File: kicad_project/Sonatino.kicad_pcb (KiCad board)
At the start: 4 copper layers, 65 x 30 mm, 129 parts, among them J2 Conn_02x09_Odd_Even, J3 USB_C_Receptacle_USB2.0, J4 Conn_01x01, J5 AudioJack4, J6 Conn_01x02, J7 Conn_01x02, Q1 DMP2104LP, Q2 DMP2104LP, Q3 HSCC8233, Q4 TPM3134NX3, Q5 DMP2104LP, SW1 SW_Push, SW2 SW_Push, SW3 SW_DIP_x02, U1 MAX98357A, U10 FSA2269, U11 TC7WH08FK,LJ(CT, U13 WM8524, U14 MAX4467, U15 WM8782, U16 TPA6132A2RTE, U2 ESP32-S3-WROOM-1U, U3 SRV05-4, U4 TP4056, U5 DW01x, U6 NCP167BMX330TBG, U7 NCP167BMX330TBG, U8 SN74LVC1G14DCKR, U9 FSA2269

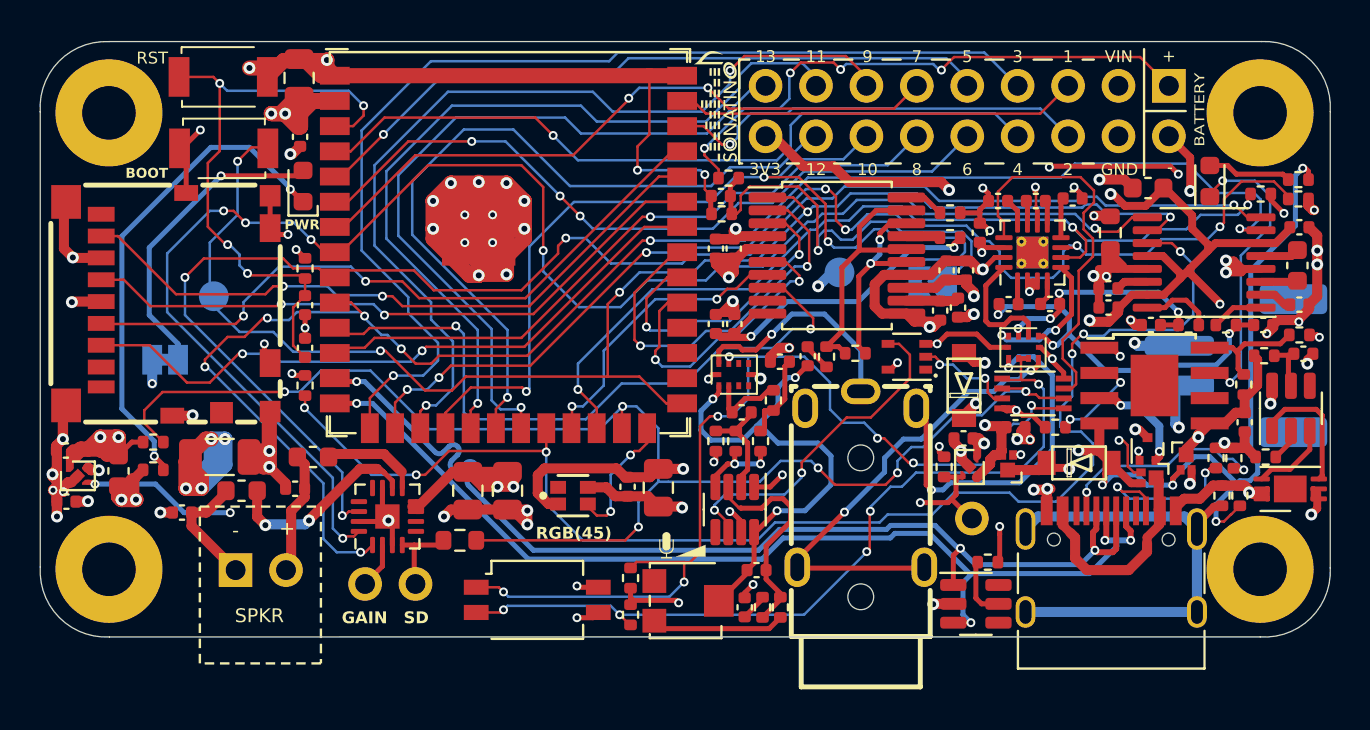
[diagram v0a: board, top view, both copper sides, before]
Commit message: Initial commit
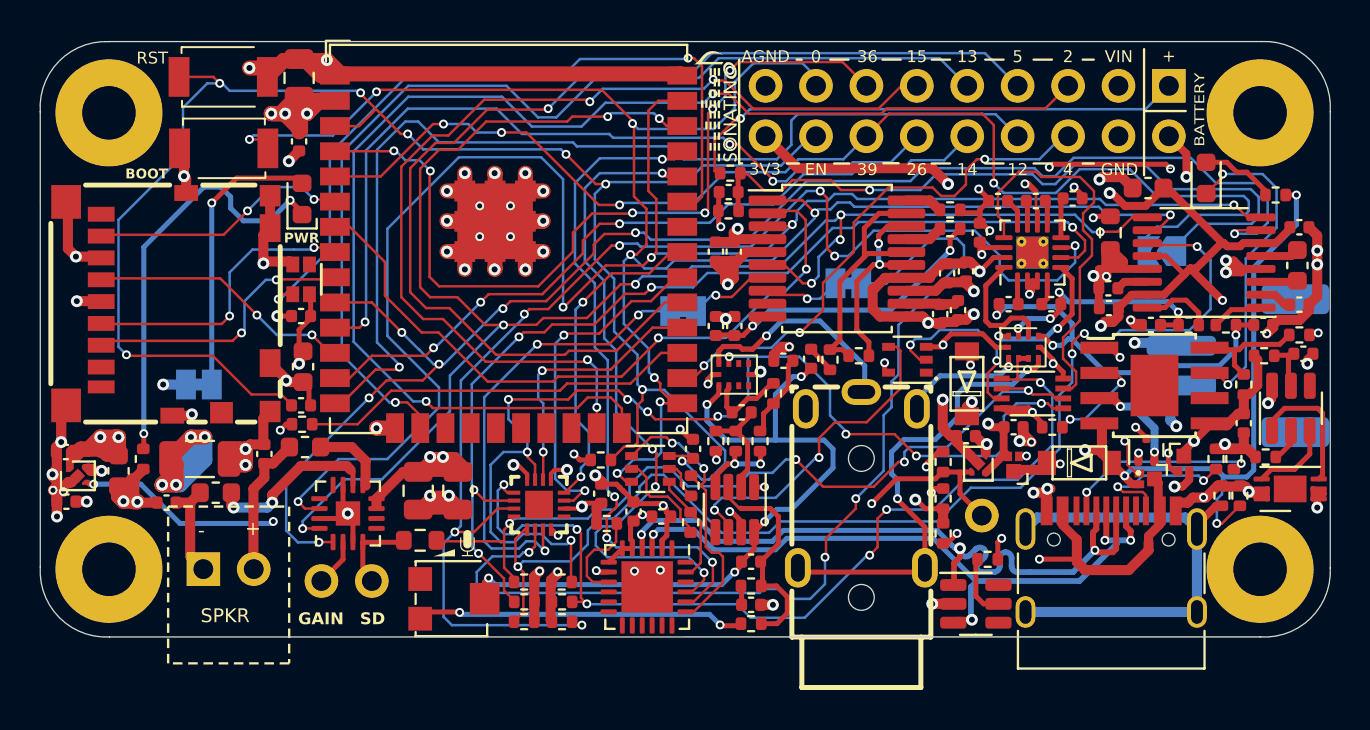
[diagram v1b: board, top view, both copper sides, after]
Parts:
- removed C47: 0.1uF, Capacitor_SMD:C_0402_1005Metric
- removed Card2: TF-008, Custom:TF-SMD_TF-008
- removed J4: Conn_01x01, Connector_PinHeader_2.54mm:PinHeader_1x01_P2.54mm_Vertical
- removed R19: 680K, Resistor_SMD:R_0603_1608Metric
- removed R4, R5, R8: 10K, Resistor_SMD:R_0402_1005Metric
- removed SW3: SW_DIP_x02, Button_Switch_SMD:SW_DIP_SPSTx02_Slide_Omron_A6H-2101_W6.15mm_P1.27mm
- removed TP1, TP2: TestPoint, TestPoint:TestPoint_Pad_D1.5mm
- added C17: 0.1uF, Capacitor_SMD:C_0402_1005Metric, F.Cu at (140.6, 46.6)
- added C48: 0.1uF, Capacitor_SMD:C_0402_1005Metric, F.Cu at (160.3, 53.3)
- added C49: 0.1uF, Capacitor_SMD:C_0402_1005Metric, F.Cu at (158.8, 56.7)
- added C50: 4.7uF, Capacitor_SMD:C_0402_1005Metric, F.Cu at (157.3, 56.5)
- added Card1: TF-008, Custom:TF-SMD_TF-008, F.Cu at (133.9, 46.0)
- added J8: Conn_01x01, Connector_PinHeader_2.54mm:PinHeader_1x01_P2.54mm_Vertical, F.Cu at (174.9, 56.7)
- added JP3: SolderJumper_2_Bridged, Jumper:SolderJumper-2_P1.3mm_Bridged_Pad1.0x1.5mm, B.Cu at (159.8, 46.4)
- added JP4: SolderJumper_2_Open, Jumper:SolderJumper-2_P1.3mm_Open_TrianglePad1.0x1.5mm, B.Cu at (184.0, 43.3)
- added Q6: MMDT3052DW 5G, Package_TO_SOT_SMD:SOT-363_SC-70-6, F.Cu at (158.2, 54.3)
- added R38: 22K, Resistor_SMD:R_0402_1005Metric, F.Cu at (172.9, 57.5)
- added R39: 47K, Resistor_SMD:R_0402_1005Metric, F.Cu at (172.9, 55.8)
- added R40: 150K, Resistor_SMD:R_0402_1005Metric, F.Cu at (162.1, 41.3)
- added R41: 470K, Resistor_SMD:R_0402_1005Metric, F.Cu at (162.2, 39.4)
- added R45: 10K, Resistor_SMD:R_0402_1005Metric, F.Cu at (151.8, 62.0)
- added R46: 10K, Resistor_SMD:R_0402_1005Metric, F.Cu at (151.8, 60.0)
- added R47: 10K, Resistor_SMD:R_0402_1005Metric, F.Cu at (153.8, 62.0)
- added R48: 10K, Resistor_SMD:R_0402_1005Metric, F.Cu at (151.8, 61.0)
- added R49: 10K, Resistor_SMD:R_0402_1005Metric, F.Cu at (153.8, 61.0)
- added R50: 10K, Resistor_SMD:R_0402_1005Metric, F.Cu at (153.7, 60.0)
- added U12: MAX98357A, Package_DFN_QFN:TQFN-16-1EP_3x3mm_P0.5mm_EP1.23x1.23mm, F.Cu at (143.0, 56.5)
- added U18: 74AHC595, Custom:X1-QFN-16-EP_L2.5-W2.5-P0.40-BL-EP1.4, F.Cu at (152.6, 56.1)
- C14: value 10uF -> 220pF; footprint Capacitor_SMD:C_0805_2012Metric -> Capacitor_SMD:C_0402_1005Metric
- C15: value 100nF -> 0.1uF; footprint Capacitor_SMD:C_0402_1005Metric -> Capacitor_SMD:C_0805_2012Metric
- C16: value 0.1uF -> 10uF
- C18: value 220pF -> 22uF; footprint Capacitor_SMD:C_0402_1005Metric -> Capacitor_SMD:C_0603_1608Metric
- C19: value 220pF -> 1uF
- C4: value 1uF -> 220pF
- C46: value 22uF -> 0.1uF; footprint Capacitor_SMD:C_0805_2012Metric -> Capacitor_SMD:C_0402_1005Metric
- JP2: value SolderJumper_2_Open -> SolderJumper_2_Bridged; footprint Jumper:SolderJumper-2_P1.3mm_Open_TrianglePad1.0x1.5mm -> Jumper:SolderJumper-2_P1.3mm_Bridged_Pad1.0x1.5mm
- Q1, Q2: footprint Custom:Diodes_DFN1411-3 -> CustomLibrary:Diodes_DFN1411-3
- Q4: value TPM3134NX3 -> DMP2104LP; footprint Package_TO_SOT_SMD:SOT-723 -> Custom:Diodes_DFN1411-3
- Q5: value DMP2104LP -> TPM3134NX3; footprint Custom:Diodes_DFN1411-3 -> Package_TO_SOT_SMD:SOT-723
- R3: value 10K -> 680K; footprint Resistor_SMD:R_0402_1005Metric -> Resistor_SMD:R_0603_1608Metric
- R34: value 150K -> 10K
- R35: value 470K -> 10K
- R37: value 100K -> 1K
- R6: value 10K -> 100K
- U1: value MAX98357A -> ESP32-WROOM-E; footprint Package_DFN_QFN:TQFN-16-1EP_3x3mm_P0.5mm_EP1.23x1.23mm -> Espressif:ESP32-WROOM-32UE
- U2: value ESP32-S3-WROOM-1U -> CP2102N-Axx-xQFN24; footprint Espressif:ESP32-S3-WROOM-1U -> Package_DFN_QFN:QFN-24-1EP_4x4mm_P0.5mm_EP2.6x2.6mm
- moved C19 31.9 mm to (162.1, 40.4)
- moved C15 21.3 mm to (146.5, 55.4), turned to -90 degrees
- moved R36 20.2 mm to (155.7, 53.9)
- moved U2 18.8 mm to (158.0, 60.2), turned to -90 degrees
- moved R7 18.2 mm to (175.2, 58.9), turned to 180 degrees
- moved D1 17.5 mm to (140.6, 44.8), turned to -90 degrees
- moved R34 17.5 mm to (160.2, 57.0), turned to 90 degrees
- moved R37 17.2 mm to (156.0, 57.0), turned to 180 degrees
- moved C14 17.2 mm to (133.8, 56.0), turned to 0 degrees
- moved R6 16.8 mm to (172.9, 54.0), turned to -90 degrees
- moved U1 15.1 mm to (151.1, 42.9), turned to 0 degrees
- moved R3 14.3 mm to (146.6, 57.9)
- moved R35 13.8 mm to (160.2, 55.1), turned to 90 degrees
- moved R28 11.8 mm to (148.2, 60.9)
- moved J7 8.18 mm to (135.7, 59.4)
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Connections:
- C14 pad 2: +5V -> Net-(J7-Pin_1)
- C15 pad 1: GND -> +5V
- C15 pad 2: Net-(JP2-A) -> GND
- C16 pad 1: +5V -> GND
- C16 pad 2: GND -> +5V
- C18 pad 1: Net-(J6-Pin_2) -> +3.3V
- C19 pad 2: Net-(J6-Pin_1) -> Net-(JP4-A)
- C4 pad 1: GND -> Net-(J7-Pin_2)
- C4 pad 2: /EN -> GND
- C46 pad 1: +3.3V -> GND
- C46 pad 2: GND -> +3.3V
- D2 pad 1: /USB & Power/VCC -> Net-(D2-K)
- D2 pad 2: Net-(D2-A) -> /VIN
- D3 pad 1: Net-(D2-A) -> /USB & Power/VCC
- D3 pad 2: /VIN -> Net-(D2-K)
- FB1 pad 1: Net-(U1-OUT-) -> Net-(U12-OUT-)
- FB1 pad 2: Net-(J6-Pin_1) -> Net-(J7-Pin_1)
- FB2 pad 1: Net-(J6-Pin_2) -> Net-(J7-Pin_2)
- FB2 pad 2: Net-(U1-OUT+) -> Net-(U12-OUT+)
- J2 pad 10: /GPIO6 -> /GPIO14
- J2 pad 11: /GPIO7 -> /GPIO15
- J2 pad 12: /GPIO8 -> /GPIO26
- J2 pad 13: /GPIO9 -> /GPIO36
- J2 pad 14: /GPIO10 -> /GPIO39
- J2 pad 15: /GPIO11 -> /BOOT/MCLK
- J2 pad 16: /GPIO12 -> /EN
- J2 pad 17: /GPIO13 -> GNDA
- J2 pad 5: /GPIO1 -> /GPIO2
- J2 pad 6: /GPIO2 -> /GPIO4
- J2 pad 7: /GPIO3 -> /GPIO5
- J2 pad 8: /GPIO4 -> /GPIO12
- J2 pad 9: /GPIO5 -> /GPIO13
- J3 pad A4: Net-(Q5-D) -> /USB & Power/VBUS
- J3 pad A6: /D+ -> /USB & Power/D+
- J3 pad A7: /D- -> /USB & Power/D-
- J3 pad A9: Net-(Q5-D) -> /USB & Power/VBUS
- J3 pad B4: Net-(Q5-D) -> /USB & Power/VBUS
- J3 pad B6: /D+ -> /USB & Power/D+
- J3 pad B7: /D- -> /USB & Power/D-
- J3 pad B9: Net-(Q5-D) -> /USB & Power/VBUS
- JP2 pad 2: /GPIO10 -> /ADC_RATE
- Q1 pad 1: Net-(D2-A) -> Net-(D2-K)
- Q4 pad 1: /USB & Power/VCC -> /VIN
- Q4 pad 2: Net-(Q4-S) -> Net-(D2-K)
- Q4 pad 3: GND -> /USB & Power/VBUS
- Q5 pad 1: /VIN -> /USB & Power/VCC
- Q5 pad 2: Net-(D2-A) -> Net-(Q5-S)
- Q5 pad 3: Net-(Q5-D) -> GND
- R12 pad 2: Net-(D2-A) -> Net-(D2-K)
- R13 pad 1: Net-(D2-A) -> Net-(D2-K)
- R2 pad 1: /~{MUTE} -> Net-(U1-GPIO16)
- R3 pad 1: +3.3V -> Net-(J6-Pin_2)
- R34 pad 1: /BAT+ -> Net-(Q6-B1)
- R34 pad 2: Net-(JP2-A) -> /USB & Power/DTR
- R35 pad 1: Net-(JP2-A) -> Net-(Q6-B2)
- R35 pad 2: GND -> /USB & Power/RTS
- R36 pad 1: Net-(D2-A) -> /EN
- R36 pad 2: Net-(U3-VP) -> +3.3V
- R37 pad 1: +5V -> Net-(U2-~{RST})
- R37 pad 2: /USB & Power/EN_REG -> +3.3V
- R6 pad 1: GND -> +5V
- R6 pad 2: /MIC_LINE_SELECT -> /USB & Power/EN_REG
- R7 pad 1: /HP_LINE_SELECT -> Net-(D2-K)
- R7 pad 2: GND -> Net-(U3-VP)
- SW2 pad 2: /MCLK -> /BOOT/MCLK
- U1 pad 1: /DAT_DAC -> GND
- U1 pad 10: Net-(U1-OUT-) -> /DAT_DAC
- U1 pad 11: GND -> /GPIO26
- U1 pad 12: (no net) -> /CLK
- U1 pad 13: (no net) -> /GPIO14
- U1 pad 14: /LRCLK_DAC -> /GPIO12
- U1 pad 16: /BCLK_DAC -> /GPIO13
- U1 pad 17: GND -> unconnected-(U1-NC-Pad17)
- U1 pad 2: Net-(J7-Pin_1) -> +3.3V
- U1 pad 3: GND -> /EN
- U1 pad 4: Net-(J7-Pin_2) -> /GPIO36
- U1 pad 5: (no net) -> /GPIO39
- U1 pad 6: (no net) -> /D0
- U1 pad 7: +5V -> /DAT_ADC
- U1 pad 8: +5V -> /CMD
- U1 pad 9: Net-(U1-OUT+) -> /D3
- U13 pad 10: /MCLK -> /BOOT/MCLK
- U13 pad 8: /LRCLK_DAC -> /LRCLK_I2S
- U13 pad 9: /BCLK_DAC -> /BCLK_I2S
- U15 pad 1: /MCLK -> /BOOT/MCLK
- U15 pad 3: /LRCLK_ADC -> /LRCLK_I2S
- U15 pad 6: /BCLK_ADC -> /BCLK_I2S
- U2 pad 1: GND -> unconnected-(U2-~{RI}/CLK-Pad1)
- U2 pad 10: /DAT_DAC -> unconnected-(U2-NC-Pad10)
- U2 pad 11: /ADC_RATE -> unconnected-(U2-~{WAKEUP}/GPIO.3-Pad11)
- U2 pad 12: /GPIO8 -> unconnected-(U2-RS485/GPIO.2-Pad12)
- U2 pad 13: /D- -> unconnected-(U2-~{RXT}/GPIO.1-Pad13)
- U2 pad 14: /D+ -> unconnected-(U2-~{TXT}/GPIO.0-Pad14)
- U2 pad 15: /GPIO3 -> unconnected-(U2-~{SUSPEND}-Pad15)
- U2 pad 16: /HP_GAIN1 -> unconnected-(U2-NC-Pad16)
- U2 pad 17: /GPIO9 -> unconnected-(U2-SUSPEND-Pad17)
- U2 pad 18: /GPIO10 -> unconnected-(U2-~{CTS}-Pad18)
- U2 pad 19: /GPIO11 -> /USB & Power/RTS
- U2 pad 2: +3.3V -> GND
- U2 pad 20: /GPIO12 -> /TXD
- U2 pad 21: /GPIO13 -> /RXD
- U2 pad 22: /~{MUTE} -> unconnected-(U2-~{DSR}-Pad22)
- U2 pad 23: /ADC_BIT_DEPTH -> /USB & Power/DTR
- U2 pad 24: /HP_GAIN0 -> unconnected-(U2-~{DCD}-Pad24)
- U2 pad 25: /~{AMP_SD} -> GND
- U2 pad 3: /EN -> /USB & Power/D+
- U2 pad 4: /GPIO4 -> /USB & Power/D-
- U2 pad 5: /GPIO5 -> +3.3V
- U2 pad 6: /GPIO6 -> +3.3V
- U2 pad 7: /GPIO7 -> +3.3V
- U2 pad 8: /BCLK_DAC -> Net-(U2-VBUS)
- U2 pad 9: /LRCLK_DAC -> Net-(U2-~{RST})
- U3 pad 1: /D- -> /USB & Power/D-
- U3 pad 3: /D+ -> /USB & Power/D+
- U4 pad 3: Net-(Q4-S) -> Net-(Q5-S)
- U4 pad 4: Net-(D2-A) -> Net-(D2-K)
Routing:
- net /BOOT/MCLK: track 0.00 -> 91.6 mm, vias 0 -> 9
- net /LRCLK_I2S: track 0.00 -> 87.4 mm, vias 0 -> 5
- net /BCLK_I2S: track 0.00 -> 84.5 mm, vias 0 -> 9
- net /BCLK_DAC: track 80.6 -> 0.00 mm, vias 6 -> 0
- net /LRCLK_DAC: track 76.1 -> 0.00 mm, vias 4 -> 0
- net /MCLK: track 74.7 -> 0.00 mm, vias 5 -> 0
- net /GPIO39: track 0.00 -> 62.1 mm, vias 0 -> 4
- net /EN: track 30.3 -> 90.0 mm, vias 4 -> 8
- net /GPIO3: track 54.3 -> 0.00 mm, vias 1 -> 0
- net Net-(D2-A): track 53.9 -> 0.00 mm, vias 7 -> 0
- net /D-: track 53.6 -> 0.00 mm, vias 3 -> 0
- net /D+: track 53.0 -> 0.00 mm, vias 4 -> 0
- net Net-(D2-K): track 0.00 -> 50.1 mm, vias 0 -> 7
- net /GPIO15: track 0.00 -> 49.9 mm, vias 0 -> 4
- net /GPIO10: track 49.3 -> 0.00 mm, vias 3 -> 0
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- removed copper zone on In1.Cu, net (none)
- removed copper zone on In2.Cu, net (none)
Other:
- board text added: "BATTERY"
- board text added: "rev BT????"
- board text removed: "1"
- board text removed: "2"
- board text removed: "AGND"
- board text removed: "DIP Switch No."
- board text removed: "Headphone"
- board text removed: "Input Level"
- board text removed: "Line"
- board text removed: "MCLK/0"
- board text removed: "Mic"
- board text removed: "ON"
- board text removed: "Output Level"
- board text removed: "RGB(45)"
- board text removed: "rev ????"
